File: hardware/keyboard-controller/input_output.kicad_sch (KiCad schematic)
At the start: 21 parts, among them J4 SYNC_IN, J5 CV_OUT, J6 GATE_OUT, J7 SYNC_OUT, Q1 2N3904, U8 LM358

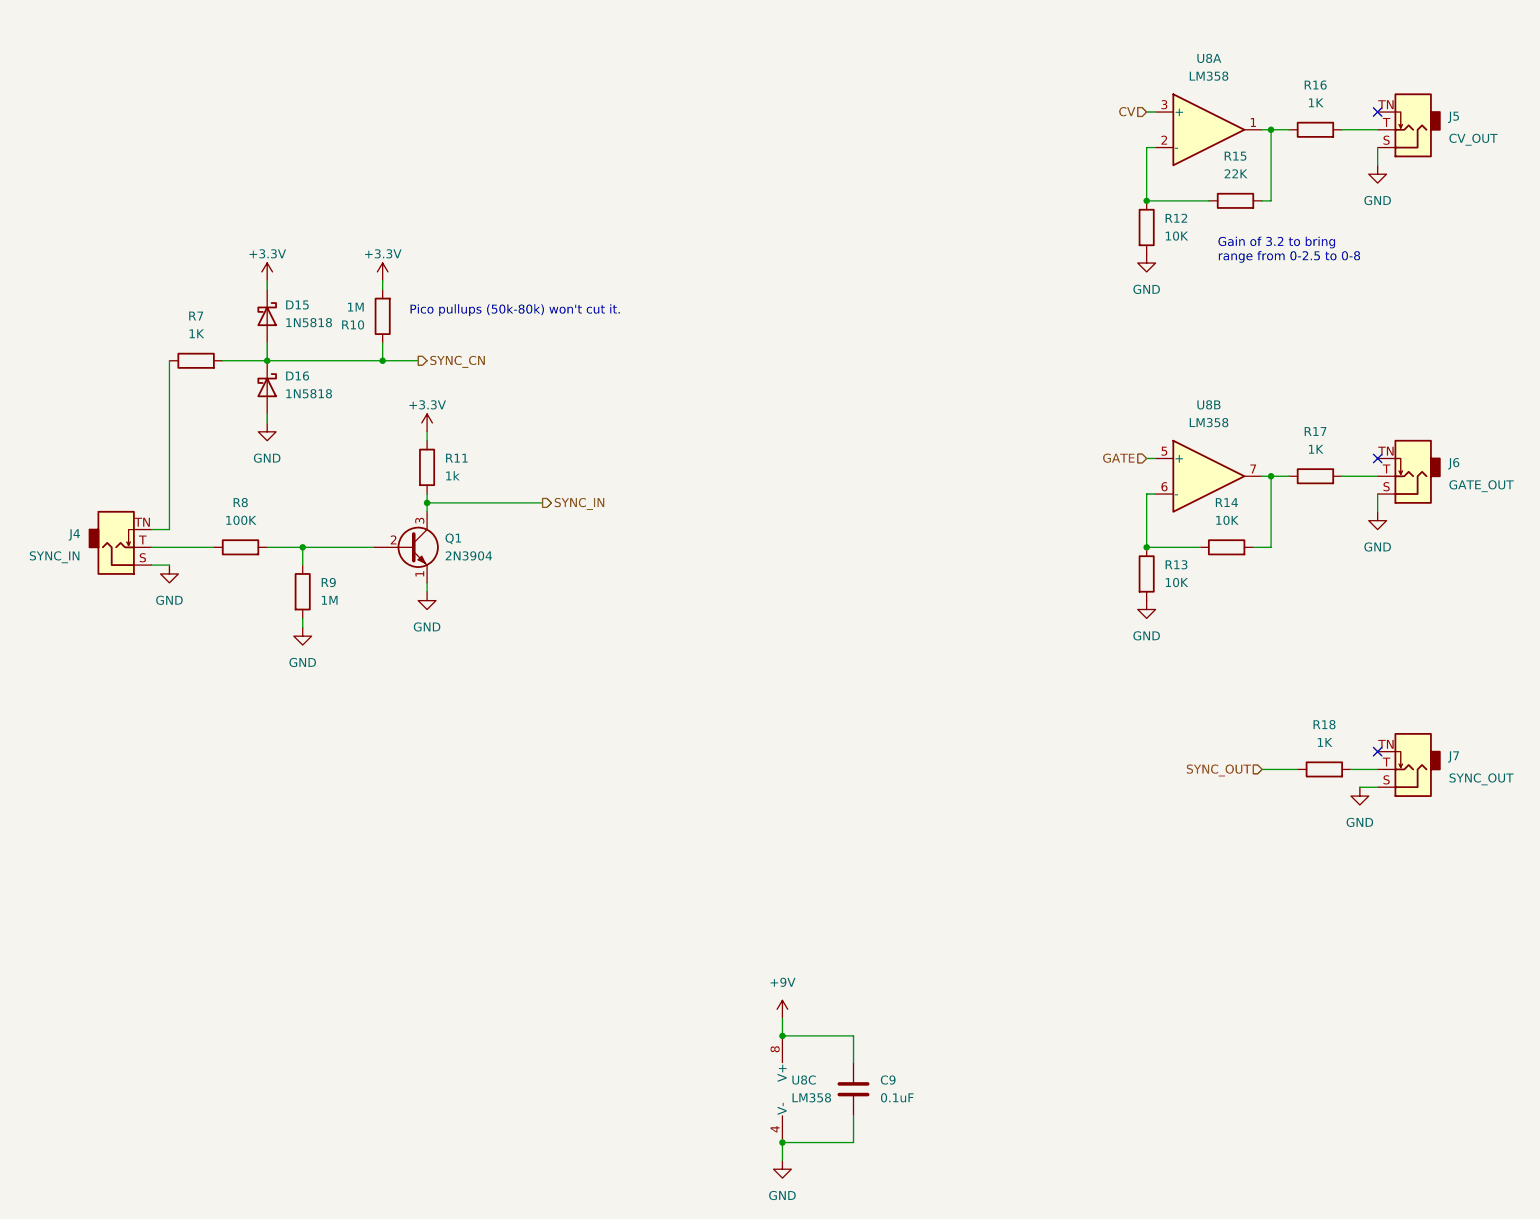
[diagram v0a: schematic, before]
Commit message: Completed initial pcb design
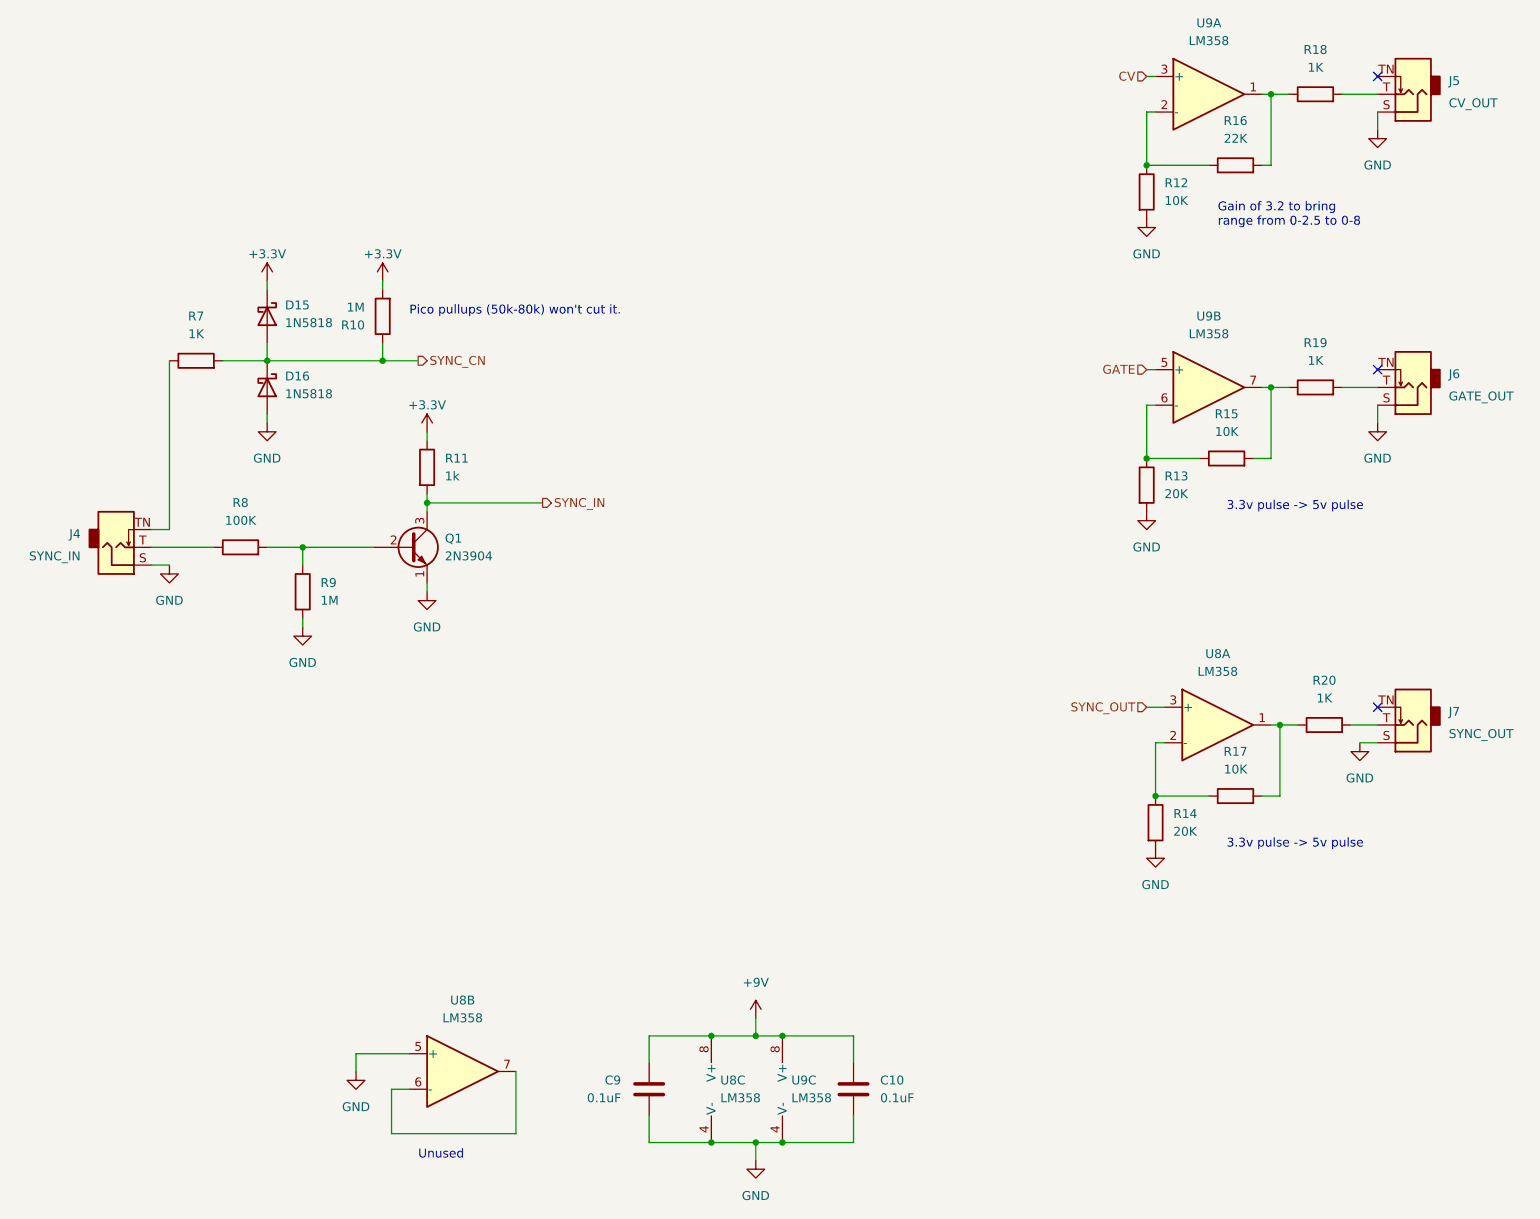
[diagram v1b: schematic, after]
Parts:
- added C9: 0.1uF, AEC_Capacitors:C_Disc_D5.0mm_W2.5mm_P3.0mm, symbol Device:C
- added R14: 20K, Royal_Ohm_Resistors:R_Axial_DIN0207_L6.8mm_D2.5mm_P10.16mm_Horizontal, symbol Device:R
- added R17: 10K, Royal_Ohm_Resistors:R_Axial_DIN0207_L6.8mm_D2.5mm_P10.16mm_Horizontal, symbol Device:R
- added U8: LM358, Package_DIP:DIP-8_W7.62mm_Socket, symbol Amplifier_Operational:LM358
- R13: value 10K -> 20K
- renumbered C9 to C10, R14 to R15, R15 to R16, R16 to R18, R17 to R19, R18 to R20, U8 to U9
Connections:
- net +9V: now also C9.1, U8.8 (V+)
- net GND: now also C9.2, R14.2, U8.4 (V-), U8.5 (+)
- net SYNC_OUT: now also U8.3 (+); no longer R20.1
- net +3V3 renamed +3.3V
- new net: R14.1, R17.1, U8.2 (-)
- new net: U8.6 (-), U8.7
- new net: R17.2, R20.1, U8.1
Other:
- note added: "3.3v pulse -> 5v pulse"
- note added: "Unused"
- moved on the sheet: J5, J6, J7, R12, R13, R15, R16, R18, R19, R20, U9A, U9B

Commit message: Added more text detail to PCB. Completed more of BOM
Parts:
- D15, D16: Manufacturer (none) -> TEC; Manufacturer Part No. (none) -> 1N5818; Supplier Part No. (none) -> A-252
- J4, J5, J6, J7: Manufacturer (none) -> Tayda; Manufacturer Part No. (none) -> PJ-629HAN-05; Supplier Part No. (none) -> A-6040
- Q1: Manufacturer (none) -> Fairchild; Manufacturer Part No. (none) -> 2N3904; Supplier Part No. (none) -> A-111
- U8: Supplier (none) -> Tayda
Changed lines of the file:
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@@
+      (effects (font (size 1.27 1.27)) hide)
+    )
+    (property "Manufacturer" "Tayda" (id 5) (at 48.26 92.71 0)
+      (effects (font (size 1.27 1.27)) hide)
+    )
+    (property "Manufacturer Part No." "PJ-629HAN-05" (id 6) (at 48.26 92.71 0)
+      (effects (font (size 1.27 1.27)) hide)
+    )
+    (property "Supplier Part No." "A-6040" (id 7) (at 48.26 92.71 0)
       (effects (font (size 1.27 1.27)) hide)
     )
@@
     )
     (property "Supplier" "Tayda" (id 4) (at 69.85 69.85 0)
+      (effects (font (size 1.27 1.27)) hide)
+    )
+    (property "Manufacturer" "TEC" (id 5) (at 69.85 69.85 0)
+      (effects (font (size 1.27 1.27)) hide)
+    )
+    (property "Manufacturer Part No." "1N5818" (id 6) (at 69.85 69.85 0)
+      (effects (font (size 1.27 1.27)) hide)
+    )
+    (property "Supplier Part No." "A-252" (id 7) (at 69.85 69.85 0)
       (effects (font (size 1.27 1.27)) hide)
     )
@@
       (effects (font (size 1.27 1.27)) hide)
     )
+    (property "Manufacturer" "Tayda" (id 5) (at 233.68 69.85 0)
+      (effects (font (size 1.27 1.27)) hide)
+    )
+    (property "Manufacturer Part No." "PJ-629HAN-05" (id 6) (at 233.68 69.85 0)
+      (effects (font (size 1.27 1.27)) hide)
+    )
+    (property "Supplier Part No." "A-6040" (id 7) (at 233.68 69.85 0)
+      (effects (font (size 1.27 1.27)) hide)
+    )
     (pin "S")
     (pin "T")
@@
     )
     (property "Datasheet" "http://www.ti.com/lit/ds/symlink/lm2904-n.pdf" (id 3) (at 97.79 167.64 0)
+      (effects (font (size 1.27 1.27)) hide)
+    )
+    (property "Supplier" "Tayda" (id 4) (at 97.79 167.64 0)
       (effects (font (size 1.27 1.27)) hide)
     )
@@
       (effects (font (size 1.27 1.27)) hide)
     )
+    (property "Manufacturer" "Tayda" (id 5) (at 233.68 27.94 0)
+      (effects (font (size 1.27 1.27)) hide)
+    )
+    (property "Manufacturer Part No." "PJ-629HAN-05" (id 6) (at 233.68 27.94 0)
+      (effects (font (size 1.27 1.27)) hide)
+    )
+    (property "Supplier Part No." "A-6040" (id 7) (at 233.68 27.94 0)
+      (effects (font (size 1.27 1.27)) hide)
+    )
     (pin "S")
     (pin "T")
@@
     )
     (property "Supplier" "Tayda" (id 4) (at 69.85 59.69 0)
+      (effects (font (size 1.27 1.27)) hide)
+    )
+    (property "Manufacturer" "TEC" (id 5) (at 69.85 59.69 0)
+      (effects (font (size 1.27 1.27)) hide)
+    )
+    (property "Manufacturer Part No." "1N5818" (id 6) (at 69.85 59.69 0)
+      (effects (font (size 1.27 1.27)) hide)
+    )
+    (property "Supplier Part No." "A-252" (id 7) (at 69.85 59.69 0)
       (effects (font (size 1.27 1.27)) hide)
     )
@@
     )
     (property "Supplier" "Tayda" (id 4) (at 233.68 118.11 0)
+      (effects (font (size 1.27 1.27)) hide)
+    )
+    (property "Manufacturer" "Tayda" (id 5) (at 233.68 118.11 0)
+      (effects (font (size 1.27 1.27)) hide)
+    )
+    (property "Manufacturer Part No." "PJ-629HAN-05" (id 6) (at 233.68 118.11 0)
+      (effects (font (size 1.27 1.27)) hide)
+    )
+    (property "Supplier Part No." "A-6040" (id 7) (at 233.68 118.11 0)
       (effects (font (size 1.27 1.27)) hide)
     )
@@
       (effects (font (size 1.27 1.27)) hide)
     )
+    (property "Manufacturer" "Fairchild" (id 5) (at 90.17 92.71 0)
+      (effects (font (size 1.27 1.27)) hide)
+    )
+    (property "Manufacturer Part No." "2N3904" (id 6) (at 90.17 92.71 0)
+      (effects (font (size 1.27 1.27)) hide)
+    )
+    (property "Supplier Part No." "A-111" (id 7) (at 90.17 92.71 0)
+      (effects (font (size 1.27 1.27)) hide)
+    )
     (pin "1")
     (pin "2")
@@
     )
     (property "Datasheet" "http://www.ti.com/lit/ds/symlink/lm2904-n.pdf" (id 3) (at 135.89 170.18 0)
+      (effects (font (size 1.27 1.27)) hide)
+    )
+    (property "Supplier" "Tayda" (id 4) (at 135.89 170.18 0)
       (effects (font (size 1.27 1.27)) hide)
     )
@@
       (effects (font (size 1.27 1.27)) hide)
     )
+    (property "Supplier" "Tayda" (id 4) (at 205.74 118.11 0)
+      (effects (font (size 1.27 1.27)) hide)
+    )
